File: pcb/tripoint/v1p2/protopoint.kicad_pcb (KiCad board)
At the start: 4 copper layers, 31.8 x 27.5 mm, 52 parts, among them T1 HHM1595A1, U1 STM32F031G6U6, U2 LXDC2HL, U3 DW1000, U4 SKY13317, U5 ProtoPoint_Module, X1 38.4M, X2 16M

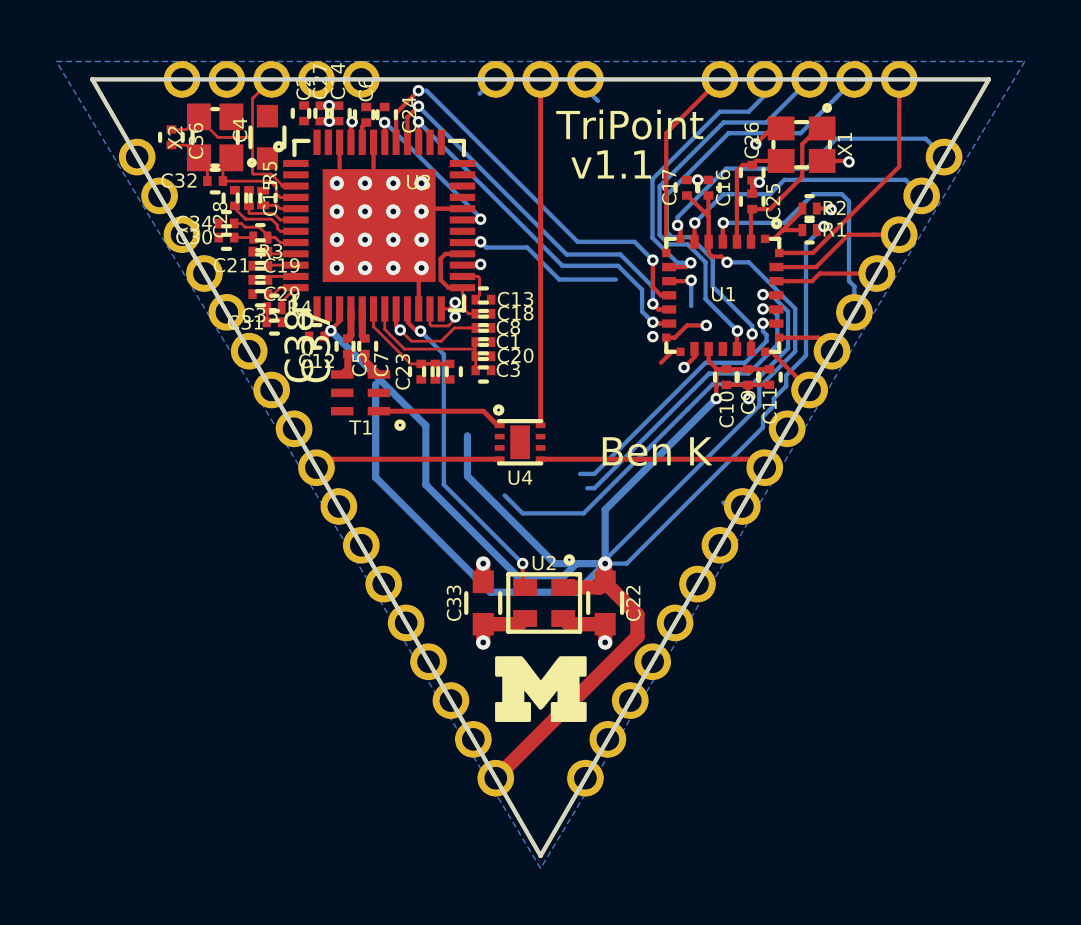
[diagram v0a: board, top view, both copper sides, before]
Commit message: done routing
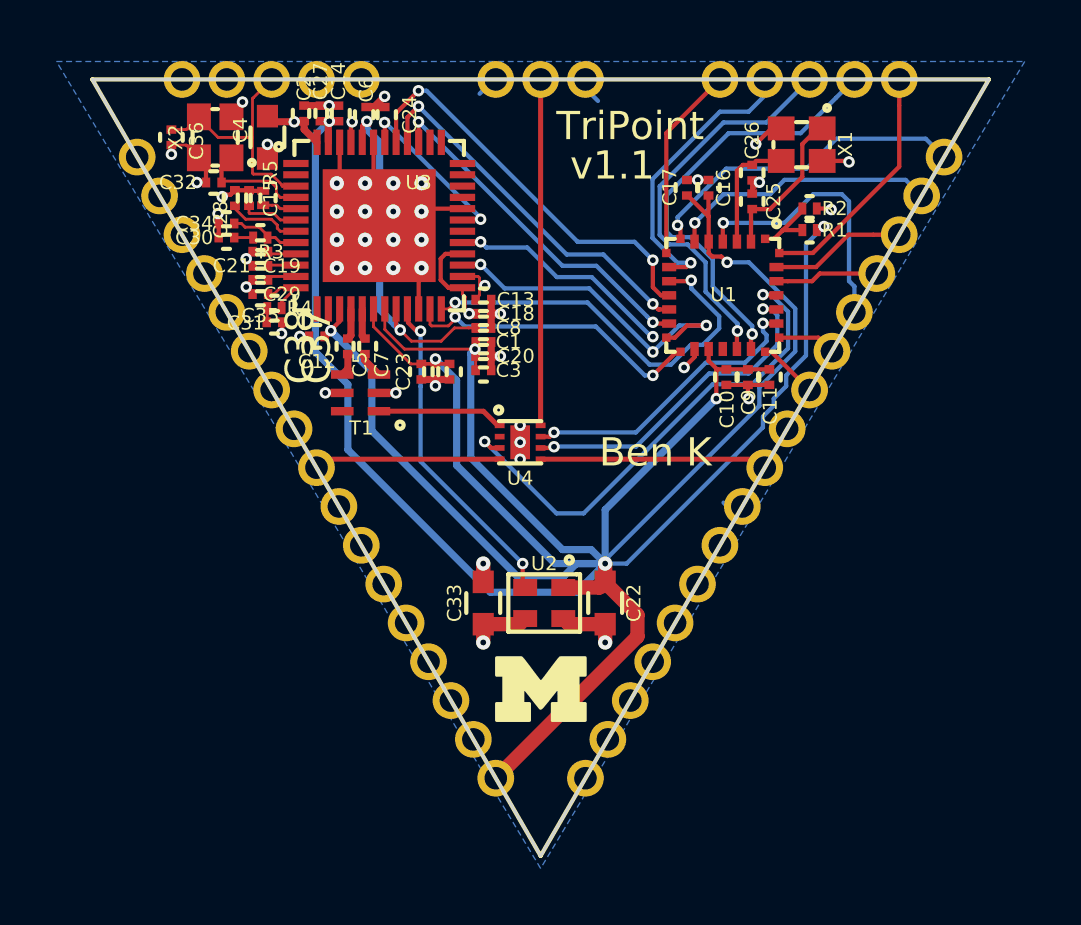
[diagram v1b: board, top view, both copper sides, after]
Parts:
- moved C32 0.07 mm to (29.7, 29.1)
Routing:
- net V3P3: track 110.4 -> 146.1 mm, vias 6 -> 9
- net GND: track 40.6 -> 57.8 mm, vias 26 -> 45
- net /DW_IRQ: track 8.04 -> 22.0 mm
- net V1P8: track 29.5 -> 42.0 mm, vias 1 -> 3
- net /~SPI1_SS: track 14.1 -> 26.1 mm
- net /~DW_RST: track 10.8 -> 20.5 mm, vias 2 -> 3
- net VDDDIG: track 4.60 -> 13.3 mm, vias 1 -> 2
- net /DW_WAKEUP: track 2.53 -> 10.9 mm, vias 1 -> 2
- net /DW_SYNC: track 21.8 -> 24.3 mm
- net /ANT_SEL0: track 15.6 -> 17.8 mm, vias 1 -> 2
- net /ANT_SEL1: track 11.0 -> 12.0 mm, vias 1 -> 2
- net /ANT_SEL2: track 9.72 -> 10.6 mm, vias 1 -> 2
- net Net-(C32-Pad1): track 3.87 -> 4.46 mm
